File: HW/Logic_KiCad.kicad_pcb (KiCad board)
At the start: 4 copper layers, 100.1 x 100 mm, 248 parts, among them J1 USB_B_Micro, Q1 Q_NPN_BEC, Q2 Q_NPN_BEC, Q4 Q_NMOS_GSD, Q5 Q_PMOS_GSD, Q6 Q_NMOS_GSD, Q7 Q_PMOS_GSD, Q8 Q_NMOS_GSD, Q9 Q_PMOS_GSD, SW1 SW_SPDT, SW10 button, SW11 button, SW12 button, SW2 button, SW3 button, SW4 button, SW5 button, SW6 button, SW7 button, SW8 button, SW9 button, U1 ESP32-PICO-D4, U2 CP2102N-A01-GQFN28, U3 SY8105

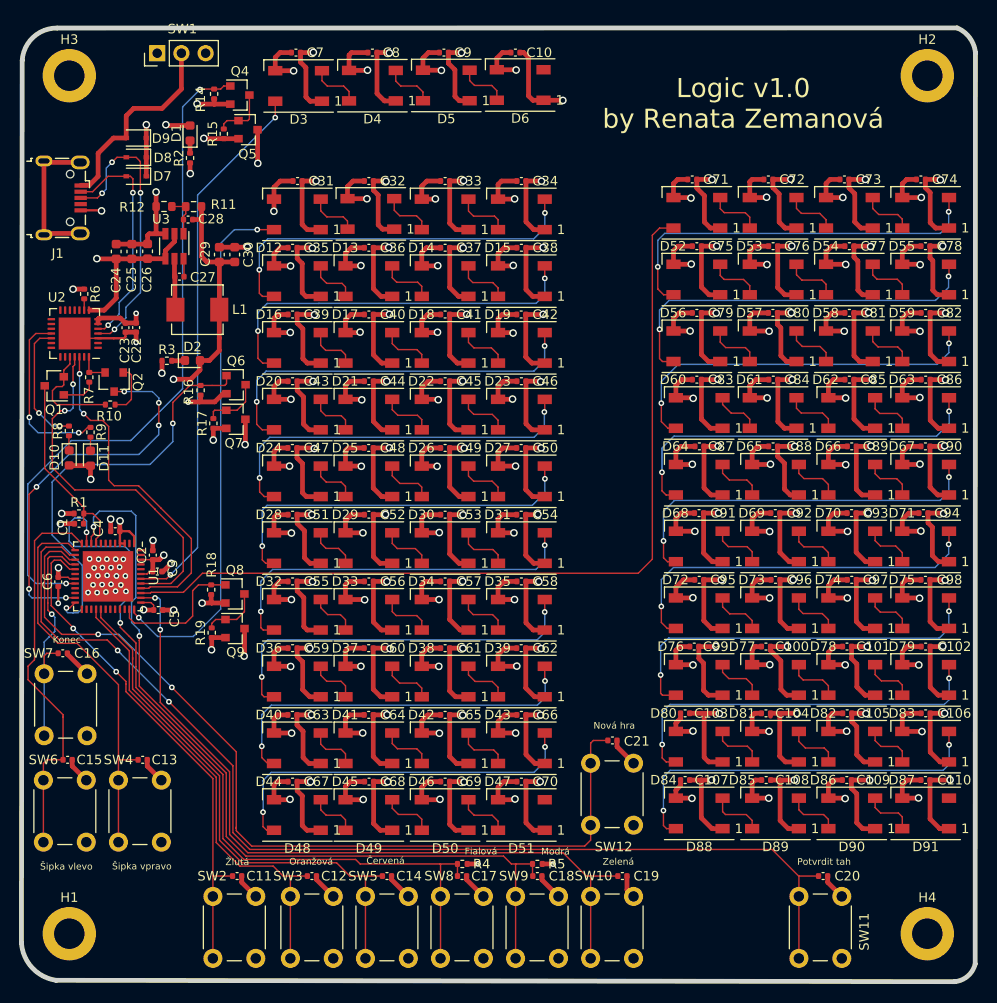
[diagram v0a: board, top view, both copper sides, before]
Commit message: v1.0 for fab
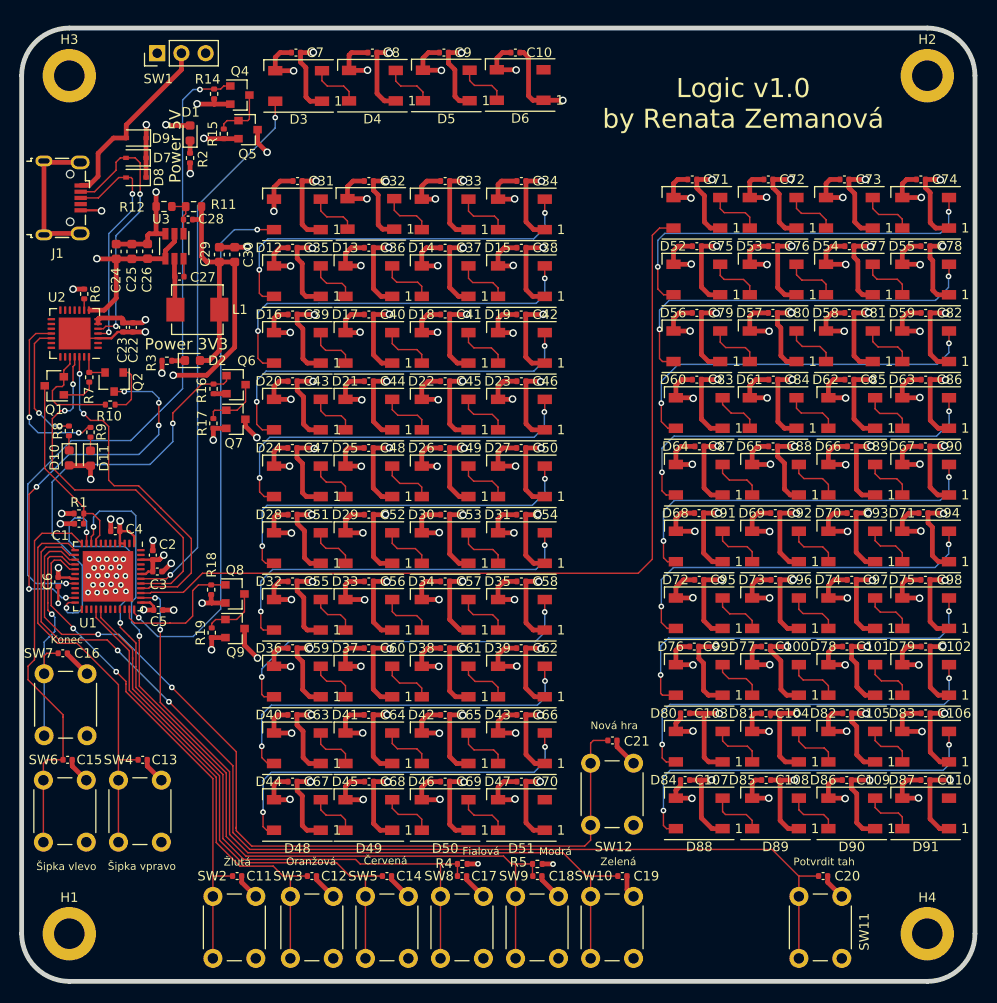
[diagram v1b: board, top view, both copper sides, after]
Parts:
- moved D8 2.12 mm to (107.0, 50.7)
- moved D7 1.93 mm to (107.0, 48.6)
- moved R16 1.37 mm to (115.1, 72.8)
- moved C22 0.34 mm to (106.7, 66.4)
- moved C23 0.26 mm to (105.6, 66.4)
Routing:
- net +3V3: track 56.4 -> 69.1 mm
- net Net-(D8-Pad2): track 30.2 -> 24.7 mm, vias 4 -> 2
- net Net-(D7-Pad2): track 23.9 -> 28.6 mm
- net GND: track 518.0 -> 514.4 mm, vias 123 -> 122
- net V_IN: track 21.3 -> 19.5 mm
- net /herni_LED.sch/8.sch/DATA_IN: track 40.2 -> 38.8 mm
- net V_LED_3: track 206.6 -> 207.4 mm
- net V_LED_1: track 302.1 -> 301.3 mm
- net ZAPINANI_2_CAST_LED: track 43.8 -> 43.2 mm
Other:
- board size 100.1 x 100 mm -> 100 x 100 mm
- board text added: "Power 3V3"
- board text added: "Power 5V"
